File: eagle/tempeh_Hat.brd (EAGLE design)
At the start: 65 x 56 mm, 8 parts, among them K1 PIN20X2

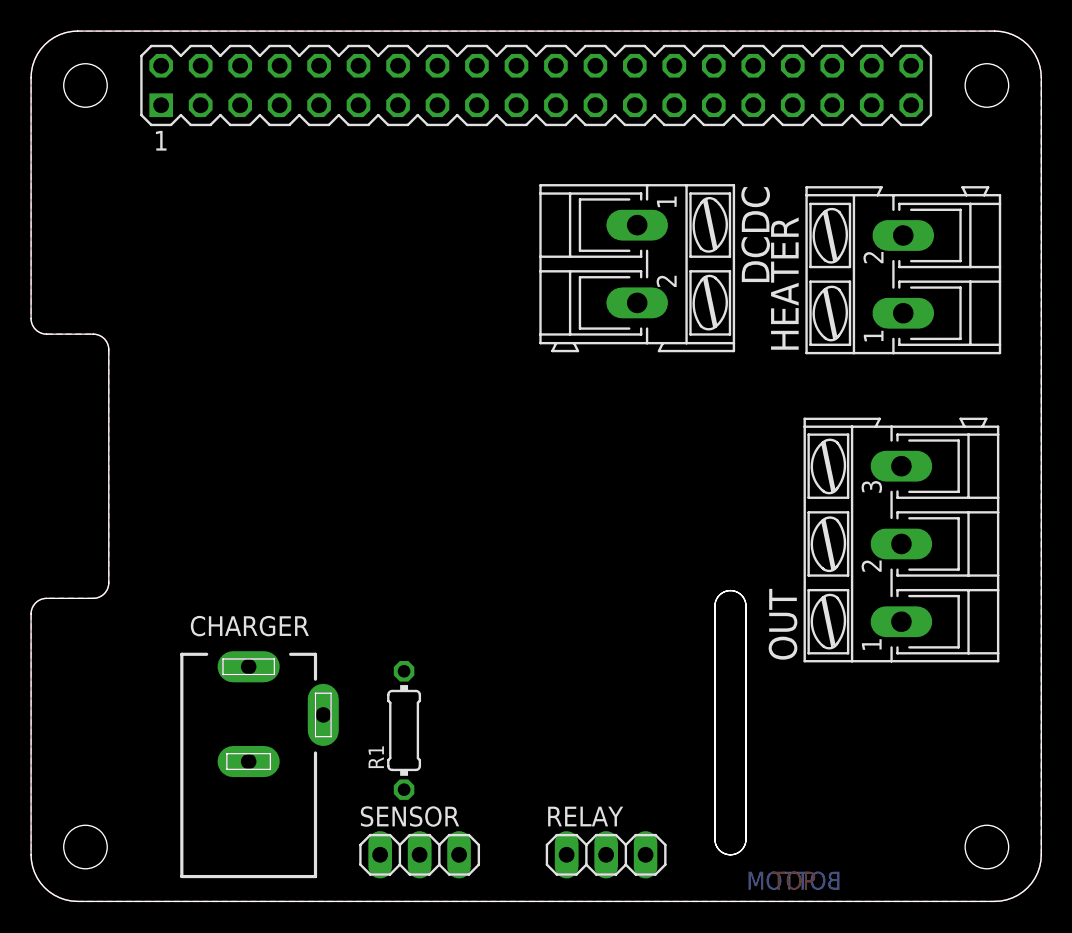
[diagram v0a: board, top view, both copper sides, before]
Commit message: adding pcb v1
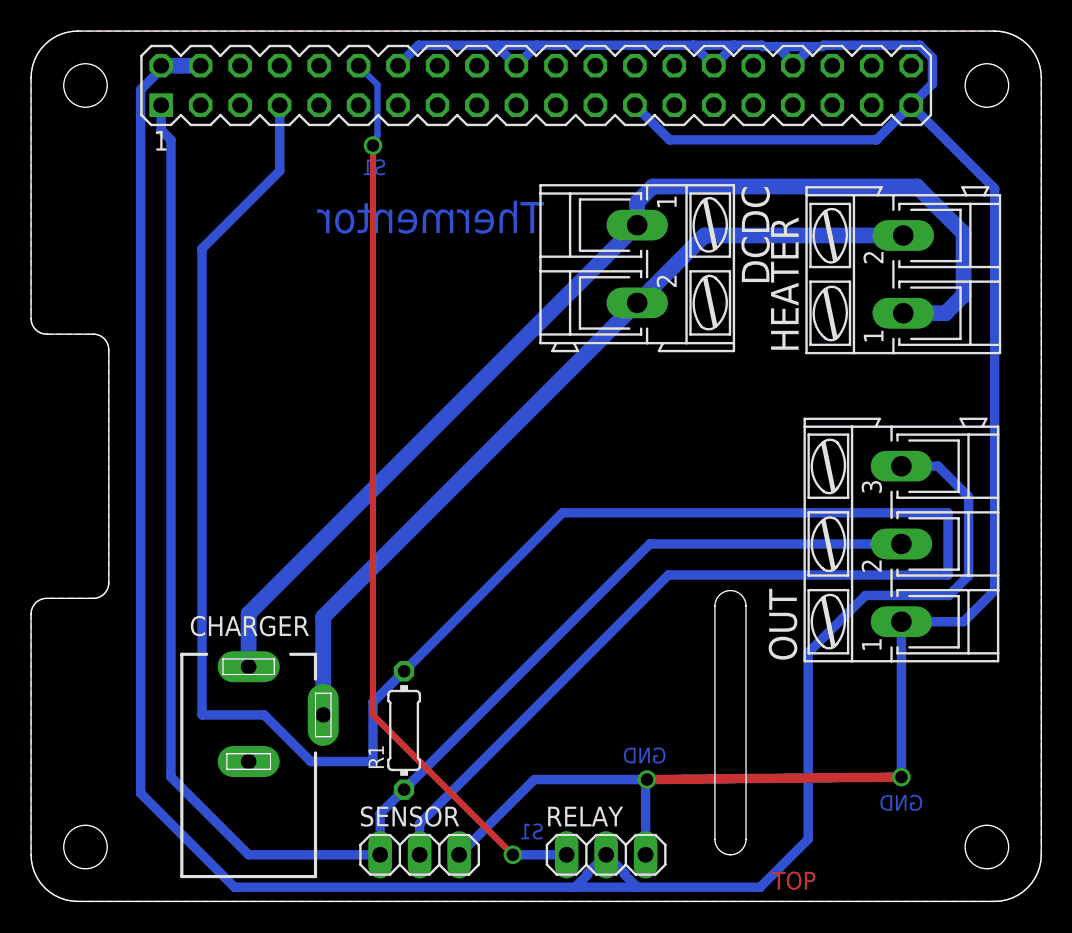
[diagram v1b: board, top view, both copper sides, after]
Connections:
- net +3V3: no longer K1.17
- net GND: no longer K1.6, K1.9
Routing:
- net GND: track 0.00 -> 155.0 mm, vias 0 -> 2
- net N$1: track 0.00 -> 146.0 mm
- net +5V: track 0.00 -> 137.0 mm
- net +3V3: track 0.00 -> 102.4 mm
- net N$5: track 0.00 -> 71.3 mm
- net N$2: track 0.00 -> 58.5 mm, vias 0 -> 3
- net N$6: track 0.00 -> 53.8 mm
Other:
- board text added: "GND"
- board text added: "S1"
- board text added: "Thermentor"
- board text removed: "BOTTOM"
